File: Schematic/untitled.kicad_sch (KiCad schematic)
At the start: 5 parts, among them U9 24LC16

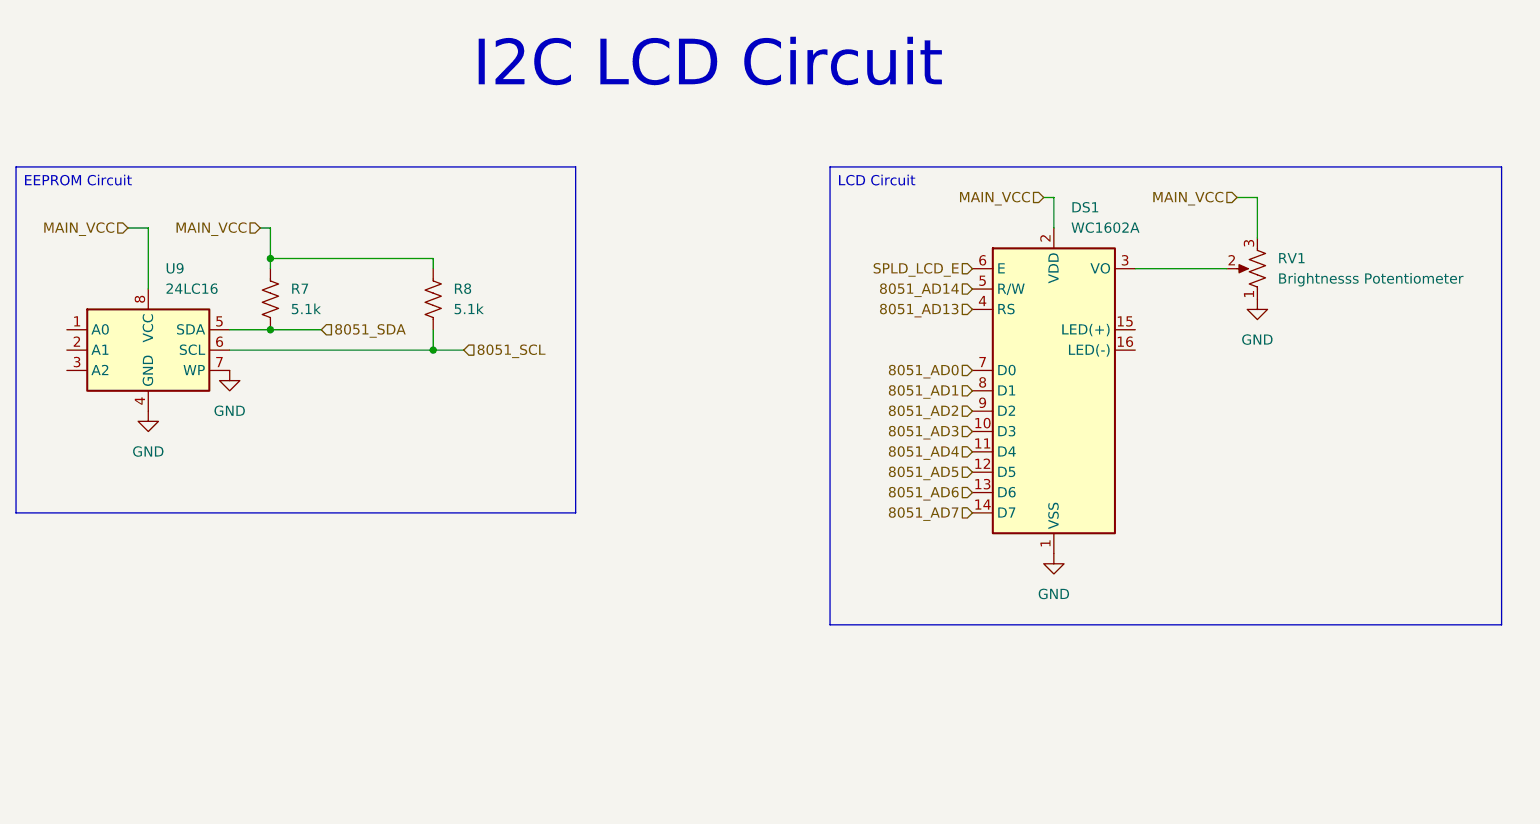
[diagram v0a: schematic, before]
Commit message: updated make and circuit
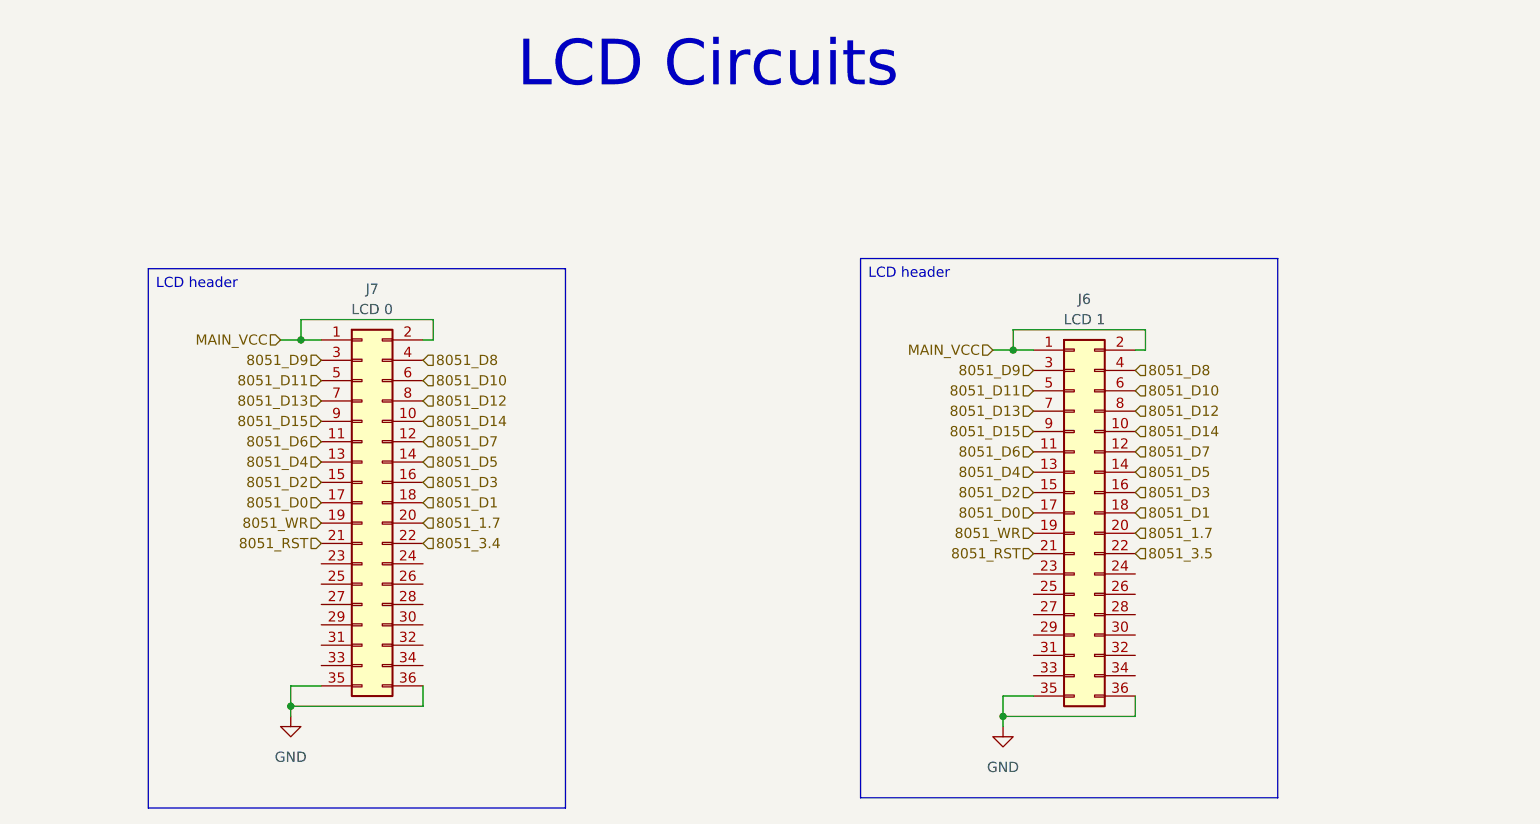
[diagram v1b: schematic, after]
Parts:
- removed DS1: WC1602A, Display:WC1602A, symbol ESD:WC1602A
- removed R7, R8: 5.1k, symbol Device:R_US
- removed RV1: Brightnesss Potentiometer, symbol Device:R_Potentiometer_US
- removed U9: 24LC16, symbol ESD:24LC16
- added J6: LCD 1, symbol Connector_Generic:Conn_02x18_Odd_Even
- added J7: LCD 0, symbol Connector_Generic:Conn_02x18_Odd_Even
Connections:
- net GND: now also J6.35 (Pin_35), J6.36 (Pin_36), J7.35 (Pin_35), J7.36 (Pin_36)
- net MAIN_VCC: now also J6.1 (Pin_1), J6.2 (Pin_2), J7.1 (Pin_1), J7.2 (Pin_2)
- new net 8051_1.7: J6.20 (Pin_20), J7.20 (Pin_20)
- new net 8051_3.4: J7.22 (Pin_22)
- new net 8051_3.5: J6.22 (Pin_22)
- new net 8051_D0: J6.17 (Pin_17), J7.17 (Pin_17)
- new net 8051_D1: J6.18 (Pin_18), J7.18 (Pin_18)
- new net 8051_D10: J6.6 (Pin_6), J7.6 (Pin_6)
- new net 8051_D11: J6.5 (Pin_5), J7.5 (Pin_5)
- new net 8051_D12: J6.8 (Pin_8), J7.8 (Pin_8)
- new net 8051_D13: J6.7 (Pin_7), J7.7 (Pin_7)
- new net 8051_D14: J6.10 (Pin_10), J7.10 (Pin_10)
- new net 8051_D15: J6.9 (Pin_9), J7.9 (Pin_9)
- new net 8051_D2: J6.15 (Pin_15), J7.15 (Pin_15)
- new net 8051_D3: J6.16 (Pin_16), J7.16 (Pin_16)
- new net 8051_D4: J6.13 (Pin_13), J7.13 (Pin_13)
- new net 8051_D5: J6.14 (Pin_14), J7.14 (Pin_14)
- new net 8051_D6: J6.11 (Pin_11), J7.11 (Pin_11)
- new net 8051_D7: J6.12 (Pin_12), J7.12 (Pin_12)
- new net 8051_D8: J6.4 (Pin_4), J7.4 (Pin_4)
- new net 8051_D9: J6.3 (Pin_3), J7.3 (Pin_3)
- new net 8051_RST: J6.21 (Pin_21), J7.21 (Pin_21)
- new net 8051_WR: J6.19 (Pin_19), J7.19 (Pin_19)
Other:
- note added: "LCD Circuits"
- note removed: "I2C LCD Circuit"
